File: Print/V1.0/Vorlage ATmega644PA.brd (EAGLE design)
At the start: 84 x 45 mm, 58 parts, among them IC1 ATmega644PA, IC4 ATTINY24/44/84-SSU, Q1 16MHz

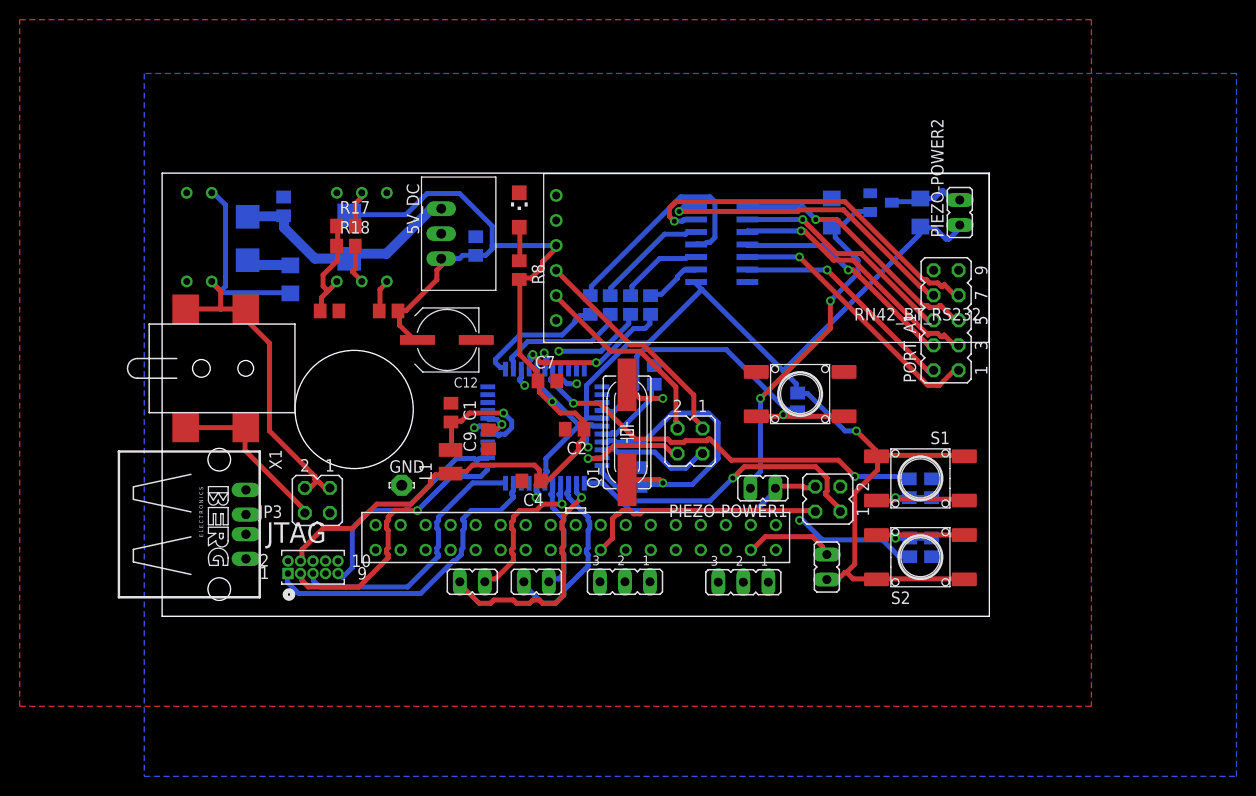
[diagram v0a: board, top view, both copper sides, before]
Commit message: printv2.0
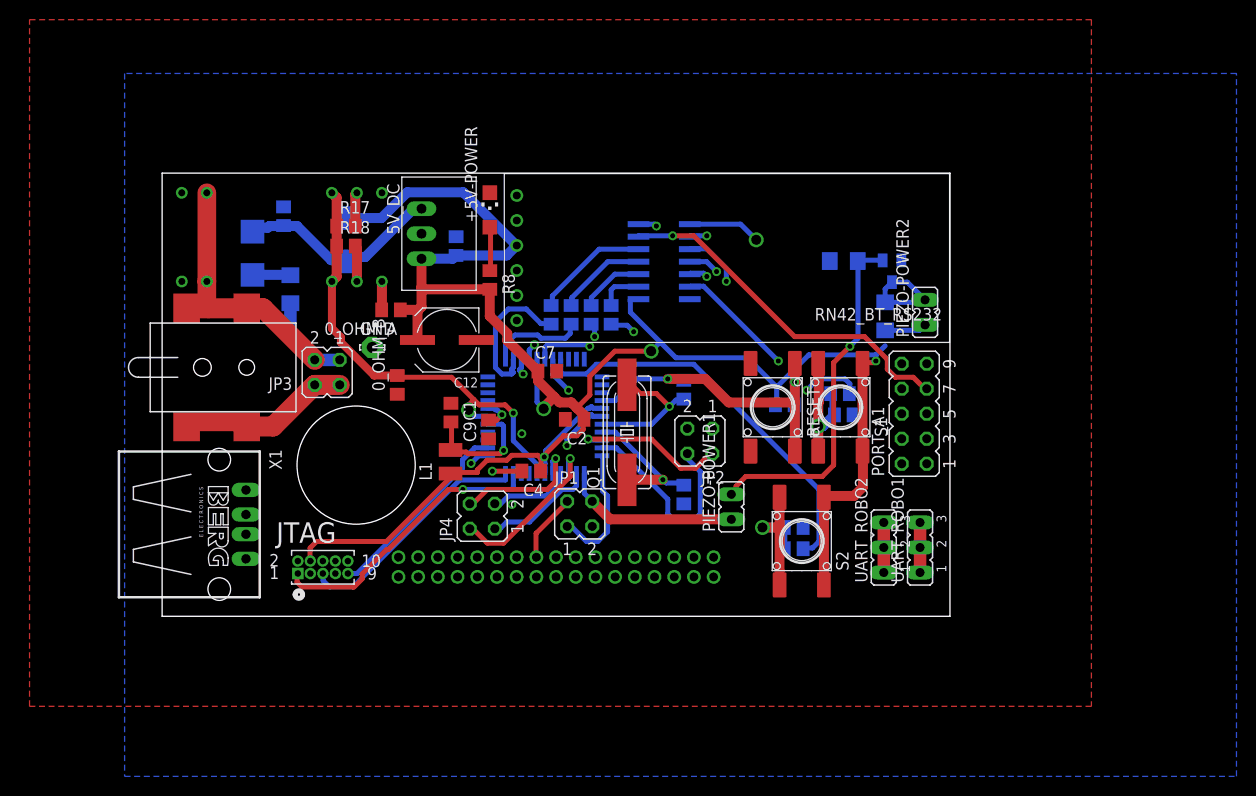
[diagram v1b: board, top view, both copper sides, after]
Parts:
- removed PIEZO-POWER3, PIEZO-POWER4, PIEZO-POWER5: (no value), jumper:JP1
- removed U$4: STECKER_2X17_2.54, untitled:2X17_2.54
- added JP4: (no value), jumper:JP2Q
- added X3: 87758-3416, con-molex:87758-3416
- moved UART_ROBO2 26.5 mm to (73.3, 6.99), turned to 90 degrees
- moved JP1 25.2 mm to (42.4, 10.4), turned to 0 degrees
- moved UART_ROBO1 18.3 mm to (77.0, 6.99), turned to 90 degrees
- moved GND 14.3 mm to (21.3, 27.3)
- moved R4 14.1 mm to (64.1, 9.02), turned to 0 degrees
- moved JP3 13.0 mm to (16.8, 24.8)
- moved S2 12.2 mm to (65.0, 7.63), turned to 90 degrees
- moved R1 11.9 mm to (68.8, 22.6), turned to 0 degrees
- moved R2 11.8 mm to (64.1, 6.86), turned to 0 degrees
- moved R3 11.6 mm to (69.2, 20.4), turned to 0 degrees
- moved R21 11.1 mm to (73.4, 30.5)
- moved S1 10.9 mm to (68.9, 21.2), turned to 90 degrees
- moved PIEZO-POWER2 10.7 mm to (77.5, 30.9)
- moved 0_OHM_B 10.2 mm to (23.9, 23.5), turned to 90 degrees
- moved PORT_A1 10.0 mm to (76.4, 20.6)
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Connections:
- new net N$10: X3.3
- new net N$11: X3.5
- new net N$19: X3.7
- new net N$2: X3.2
- new net N$20: X3.9
- new net N$29: X3.11
- new net N$33: X3.13
- new net N$41: X3.15
- new net N$47: X3.19
- new net N$52: X3.21
- new net N$53: X3.23
- new net N$54: X3.25
- new net N$55: X3.27
- new net N$56: X3.29
- new net N$57: X3.31
- new net N$58: X3.32
- new net N$65: X3.30
- new net N$67: X3.28
- new net N$68: X3.26
- new net N$69: X3.24
- new net N$71: X3.22
- new net N$73: X3.18
- new net N$74: X3.16
- new net N$76: X3.14
- new net N$77: X3.12
- new net N$78: X3.10
- new net N$79: X3.8
- new net N$80: X3.6
- new net N$82: X3.34
- new net N$83: X3.33
- net GND: now also X3.4
- net N$1: now also X3.1; no longer PIEZO-POWER4.2, U$4.32
- net PD4: now also JP4.1; no longer PIEZO-POWER3.1
- net PD5: now also JP4.2; no longer PIEZO-POWER5.2
- net PD6: now also JP4.3; no longer PIEZO-POWER3.2
- net PD7: now also JP4.4; no longer PIEZO-POWER5.1
- net RX: now also X3.17; no longer U$4.17
- net TX: now also X3.20; no longer U$4.20
- net VCC: no longer PIEZO-POWER4.1
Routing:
- net DGND: track 37.8 -> 81.1 mm
- net +5V: track 3.37 -> 37.6 mm
- net TX: track 61.3 -> 28.8 mm
- net VCC: track 232.0 -> 199.7 mm, vias 2 -> 4
- net PD2: track 30.9 -> 13.1 mm, vias 1 -> 0
- net N$36: track 30.3 -> 14.2 mm
- net +12V: track 52.3 -> 36.3 mm
- net N$3: track 23.3 -> 9.10 mm
- net PD4: track 25.1 -> 11.3 mm, vias 1 -> 0
- net RX: track 62.0 -> 50.3 mm
- net N$1: track 9.31 -> 0.00 mm
- net PD1: track 11.4 -> 20.7 mm, vias 1 -> 0
- net GND: track 0.00 -> 8.21 mm, vias 0 -> 3
- net PD3: track 26.0 -> 18.0 mm
- net PB0: track 42.1 -> 34.1 mm
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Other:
- board size 84 x 45 mm -> 80 x 45 mm
